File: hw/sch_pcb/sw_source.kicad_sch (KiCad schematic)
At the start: 31 parts, among them U1 TPS631000DRLR

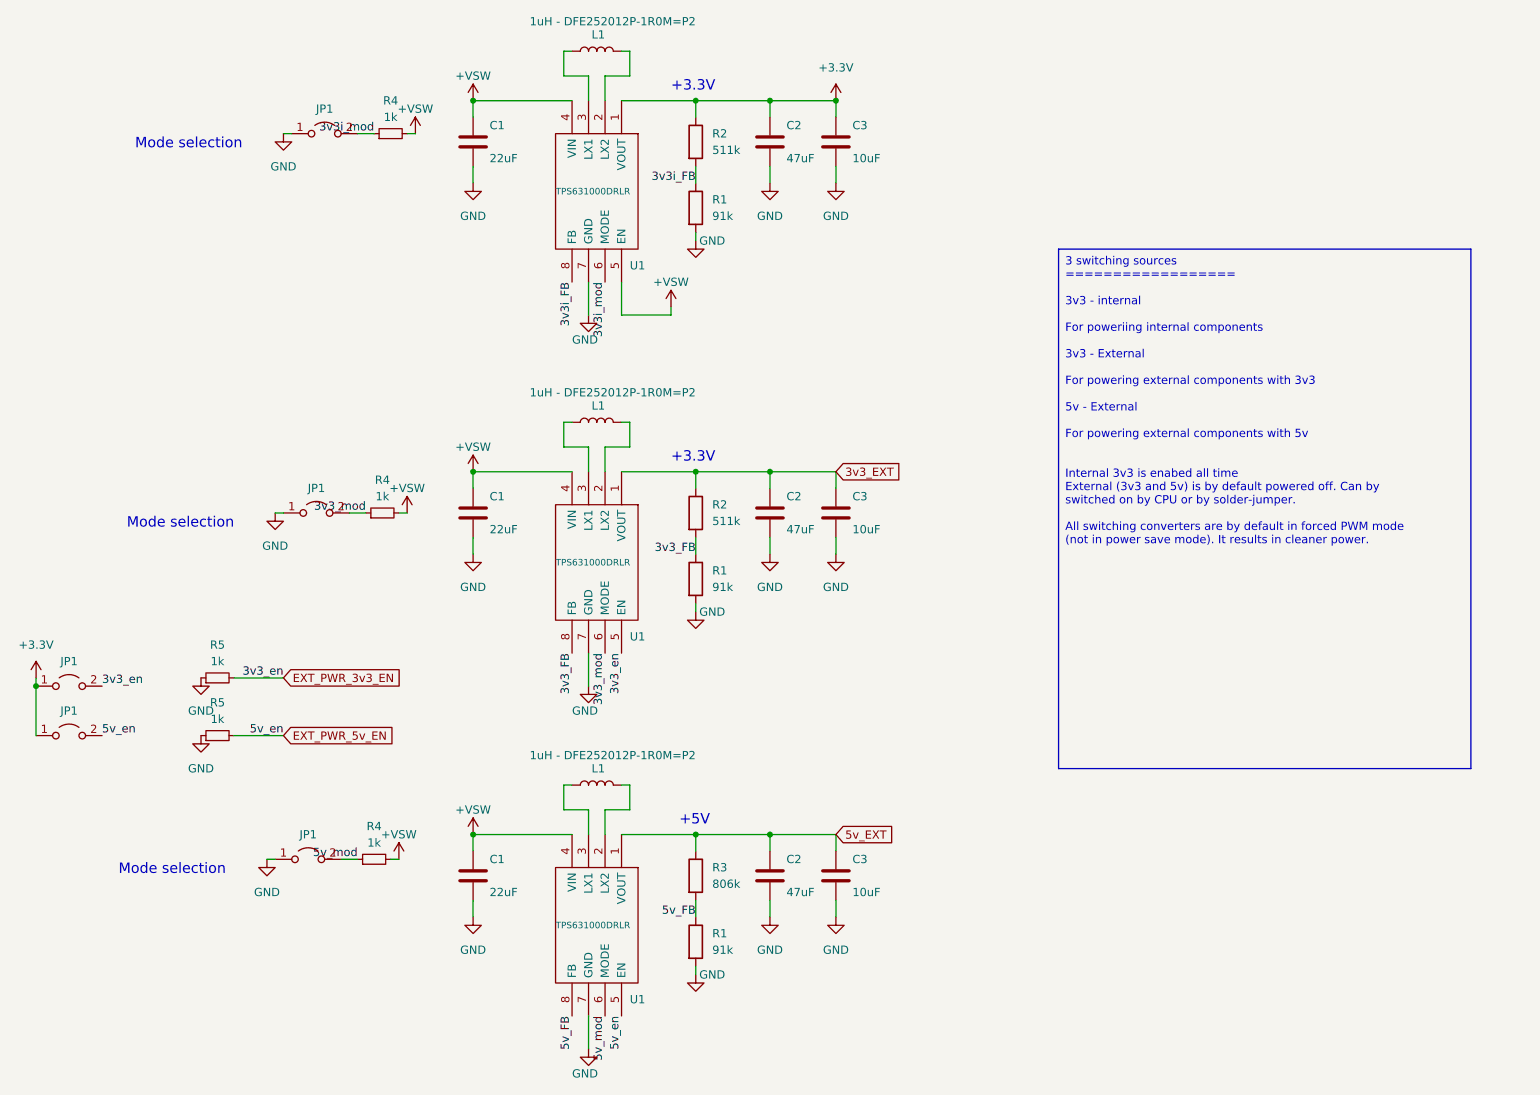
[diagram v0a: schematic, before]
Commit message: wip, update schematics, board outlines
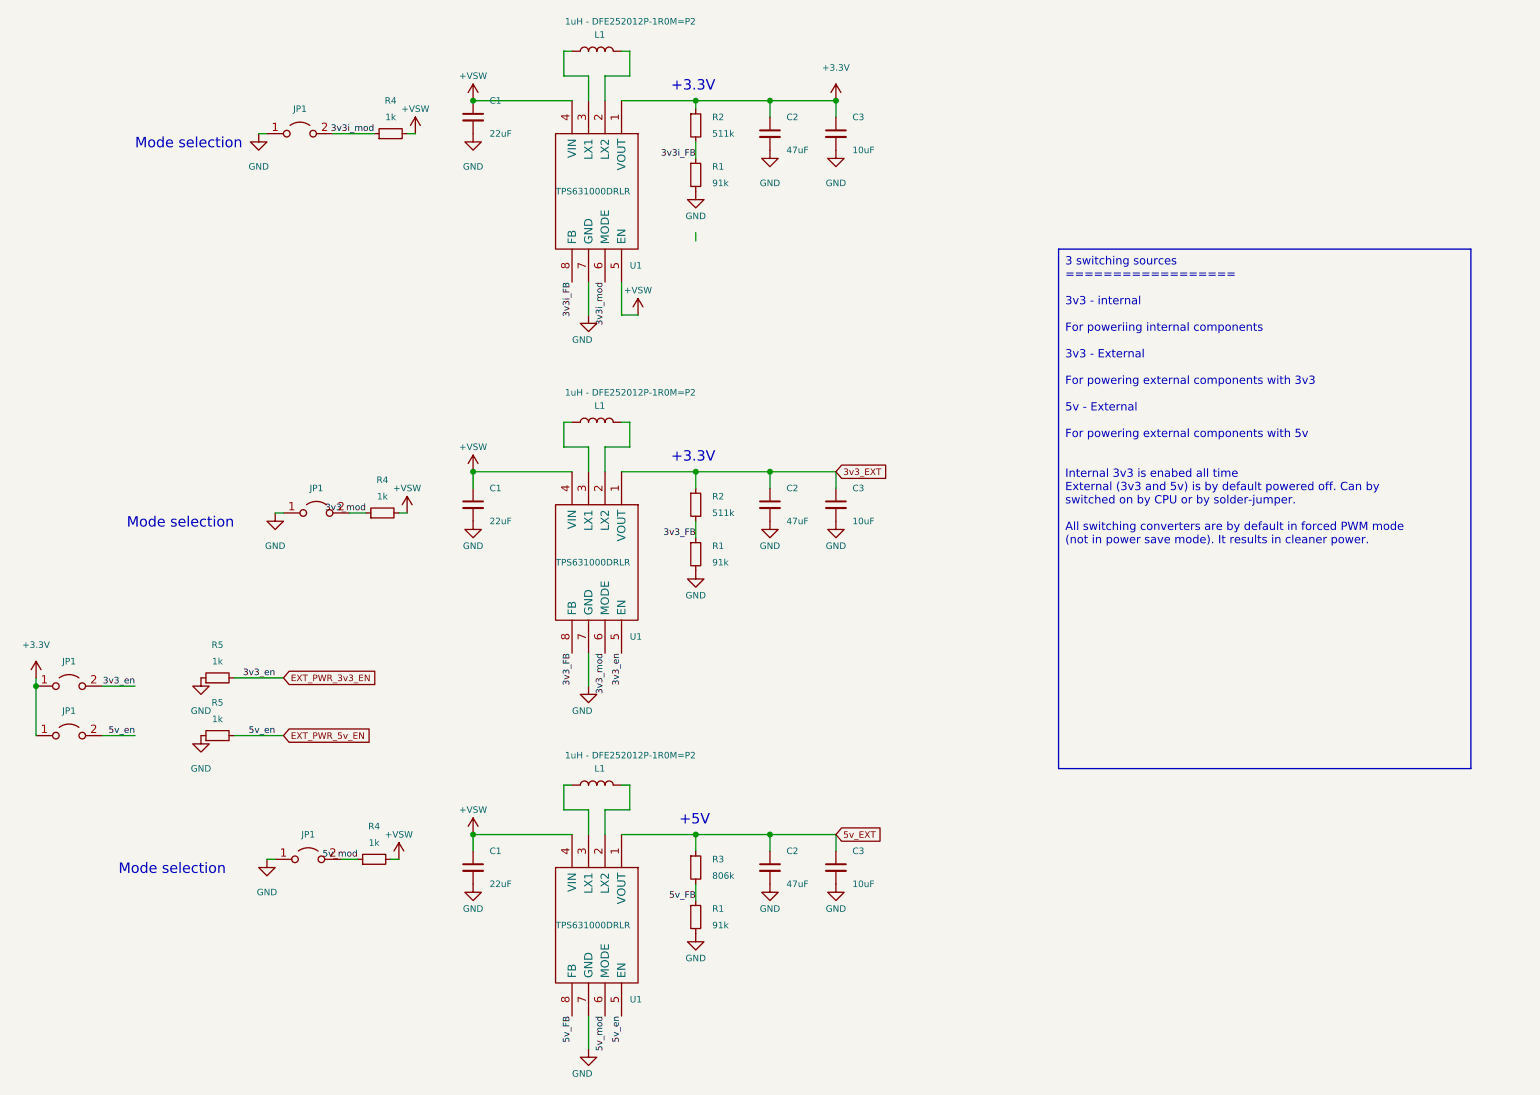
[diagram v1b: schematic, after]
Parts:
- C1: symbol Device:C -> Device:C_Small; UST_ID 650b58f1462c6d9e7205463b -> (none)
- C2: symbol Device:C -> Device:C_Small; UST_ID 5c70984812875079b91f8bbf -> (none)
- C3: symbol Device:C -> Device:C_Small; UST_ID 5c70984712875079b91f8b53 -> (none)
- R1: symbol Device:R -> Device:R_Small; UST_ID 650b59ec462c6d9e72054677 -> (none)
- R1: footprint Resistor_SMD:R_0603_1608Metric -> Resistor_SMD:R_0805_2012Metric; symbol Device:R -> Device:R_Small; UST_ID 650b59ec462c6d9e72054677 -> (none)
- R2: footprint Resistor_SMD:R_0603_1608Metric -> Resistor_SMD:R_0805_2012Metric; symbol Device:R -> Device:R_Small; UST_ID 650b5a43462c6d9e7205468e -> (none)
- R2: symbol Device:R -> Device:R_Small; UST_ID 650b5a43462c6d9e7205468e -> (none)
- R3: symbol Device:R -> Device:R_Small; UST_ID 650b5abb462c6d9e720546b8 -> (none)
- R4: footprint Resistor_SMD:R_0603_1608Metric -> Resistor_SMD:R_0805_2012Metric
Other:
- moved on the sheet: C1, C2, C3, JP1, R1, R2, R3
